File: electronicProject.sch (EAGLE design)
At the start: 18 parts, among them IC1 PIC16F877P, IC2 MAX232

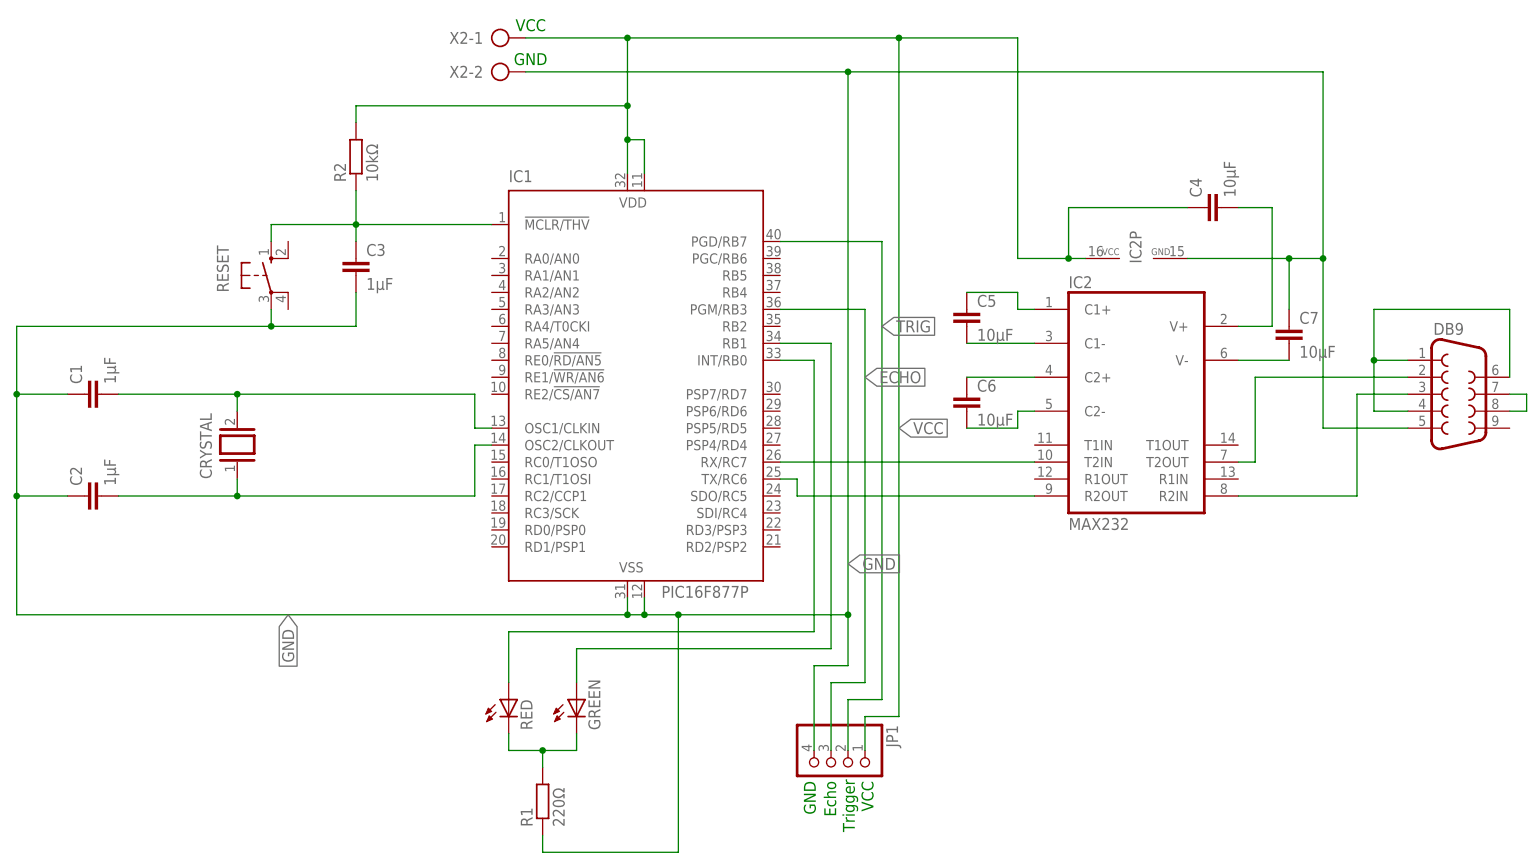
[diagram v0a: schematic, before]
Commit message: Routing
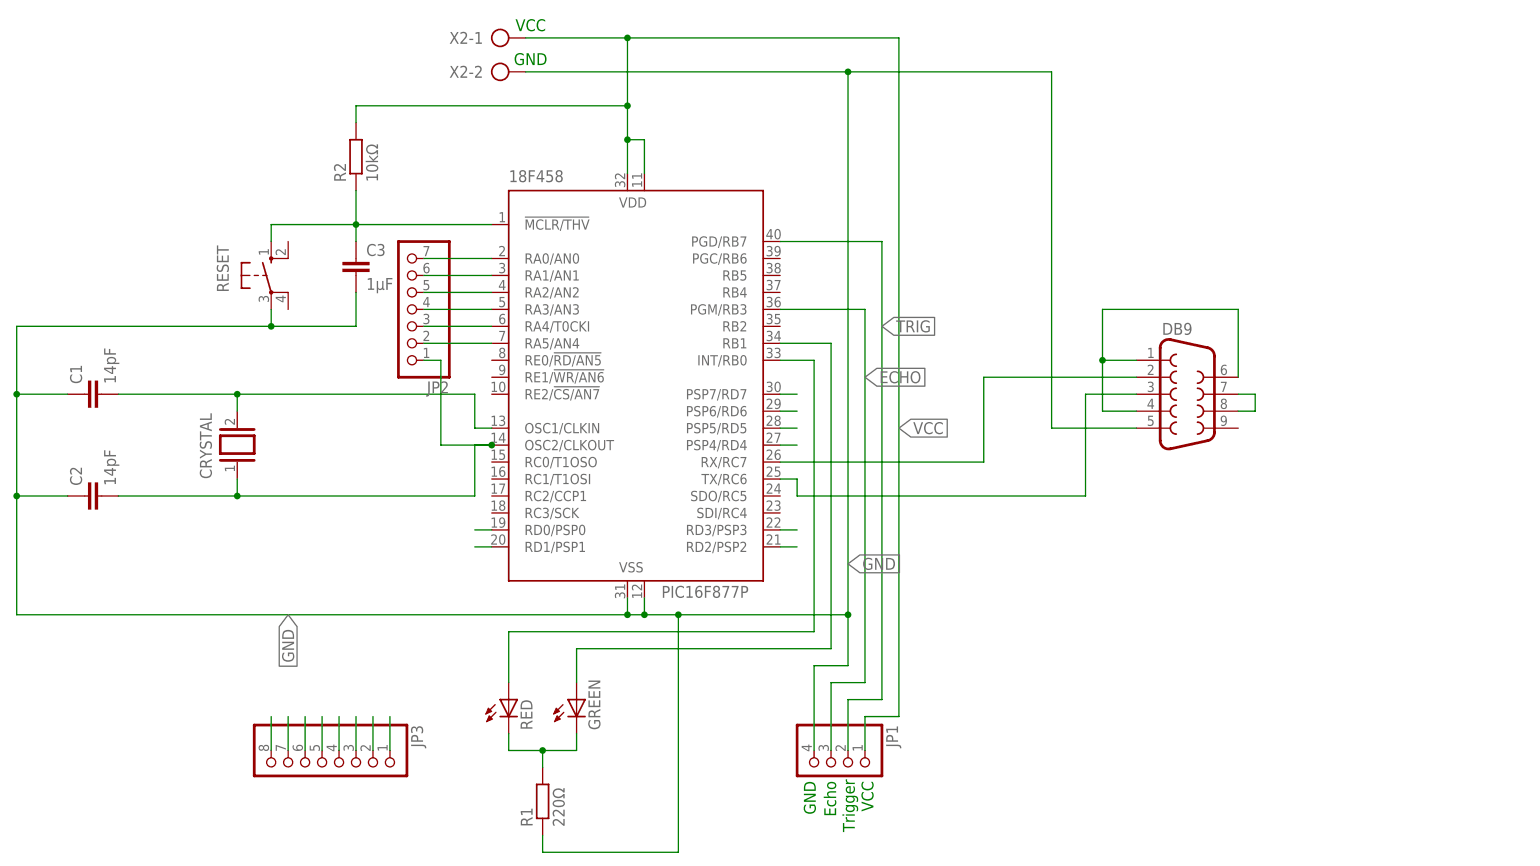
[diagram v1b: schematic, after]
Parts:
- removed C4, C5, C6, C7: 10µF, rcl:C-EU025-025X050
- removed IC2: MAX232, maxim:MAX232
- added JP2: (no value), pinhead:PINHD-1X7
- added JP3: (no value), pinhead:PINHD-1X8
- C1, C2: value 1µF -> 14pF; device rcl:C-EU025-025X050 -> rcl:C-EU025-024X044
- C3: device rcl:C-EU025-025X050 -> rcl:C-EU025-024X044
- R1, R2: device rcl:R-EU_0204/5 -> rcl:R-EU_0207/10
- renumbered IC1 to 18F458
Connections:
- removed net N$13: 18F458.OSC2/CLKOUT, C2.2, CRYSTAL.1
- removed net N$18 (its old number): C7.2, IC2G$1.V-
- removed net N$19: DB9.3, IC2G$1.R2IN
- new net N$5: 18F458.RA1/AN1, JP2.6
- new net RD0: 18F458.RD0/PSP0, JP3.8
- new net RD1: 18F458.RD1/PSP1, JP3.7
- new net RD2: 18F458.RD2/PSP2, JP3.6
- new net RD3: 18F458.RD3/PSP3, JP3.5
- new net RD4: 18F458.PSP4/RD4, JP3.4
- new net RD5: 18F458.PSP5/RD5, JP3.3
- new net RD6: 18F458.PSP6/RD6, JP3.2
- new net RD7: 18F458.PSP7/RD7, JP3.1
- net GND: no longer C7.1, IC2P.GND
- net N$10: now also 18F458.RA3/AN3, JP2.4; no longer DB9.2, IC2G$1.T2OUT
- net N$11: now also DB9.3; no longer IC2G$1.R2OUT
- net N$14: now also 18F458.RA4/T0CKI, JP2.3; no longer C5.2, IC2G$1.C1-
- net N$15: now also 18F458.RA5/AN4, JP2.2; no longer C6.1, IC2G$1.C2+
- net N$17: now also 18F458.OSC2/CLKOUT, C2.2, CRYSTAL.1, JP2.1; no longer C6.2, IC2G$1.C2-
- net N$4: now also 18F458.RA0/AN0, JP2.7; no longer C5.1, IC2G$1.C1+
- net N$6: now also 18F458.RA2/AN2, JP2.5; no longer C4.2, IC2G$1.V+
- net N$8: now also DB9.2; no longer IC2G$1.T2IN
- net VCC: no longer C4.1, IC2P.VCC
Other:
- moved on the sheet: DB9

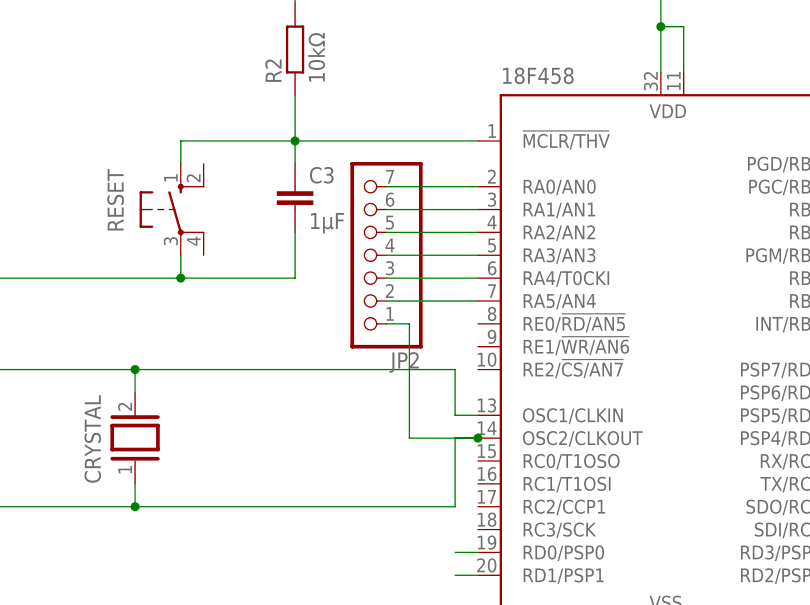
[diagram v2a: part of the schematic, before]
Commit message: final design
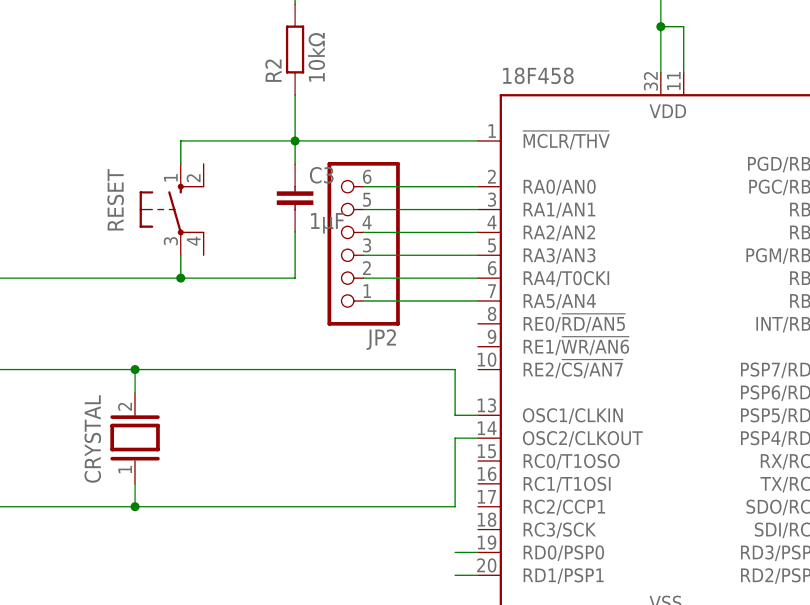
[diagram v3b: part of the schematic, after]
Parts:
- JP2: device pinhead:PINHD-1X7 -> pinhead:PINHD-1X6
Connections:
- net N$10: now also JP2.3; no longer JP2.4
- net N$14: now also JP2.2; no longer JP2.3
- net N$15: now also JP2.1; no longer JP2.2
- net N$17: no longer JP2.1
- net N$4: now also JP2.6; no longer JP2.7
- net N$5: now also JP2.5; no longer JP2.6
- net N$6: now also JP2.4; no longer JP2.5
